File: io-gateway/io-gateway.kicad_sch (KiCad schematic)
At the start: 8 parts, among them J1 1752201, J2 1752201, J3 1752201, J4 Screw_Terminal_01x09, J5 Screw_Terminal_01x09, J6 Screw_Terminal_01x09

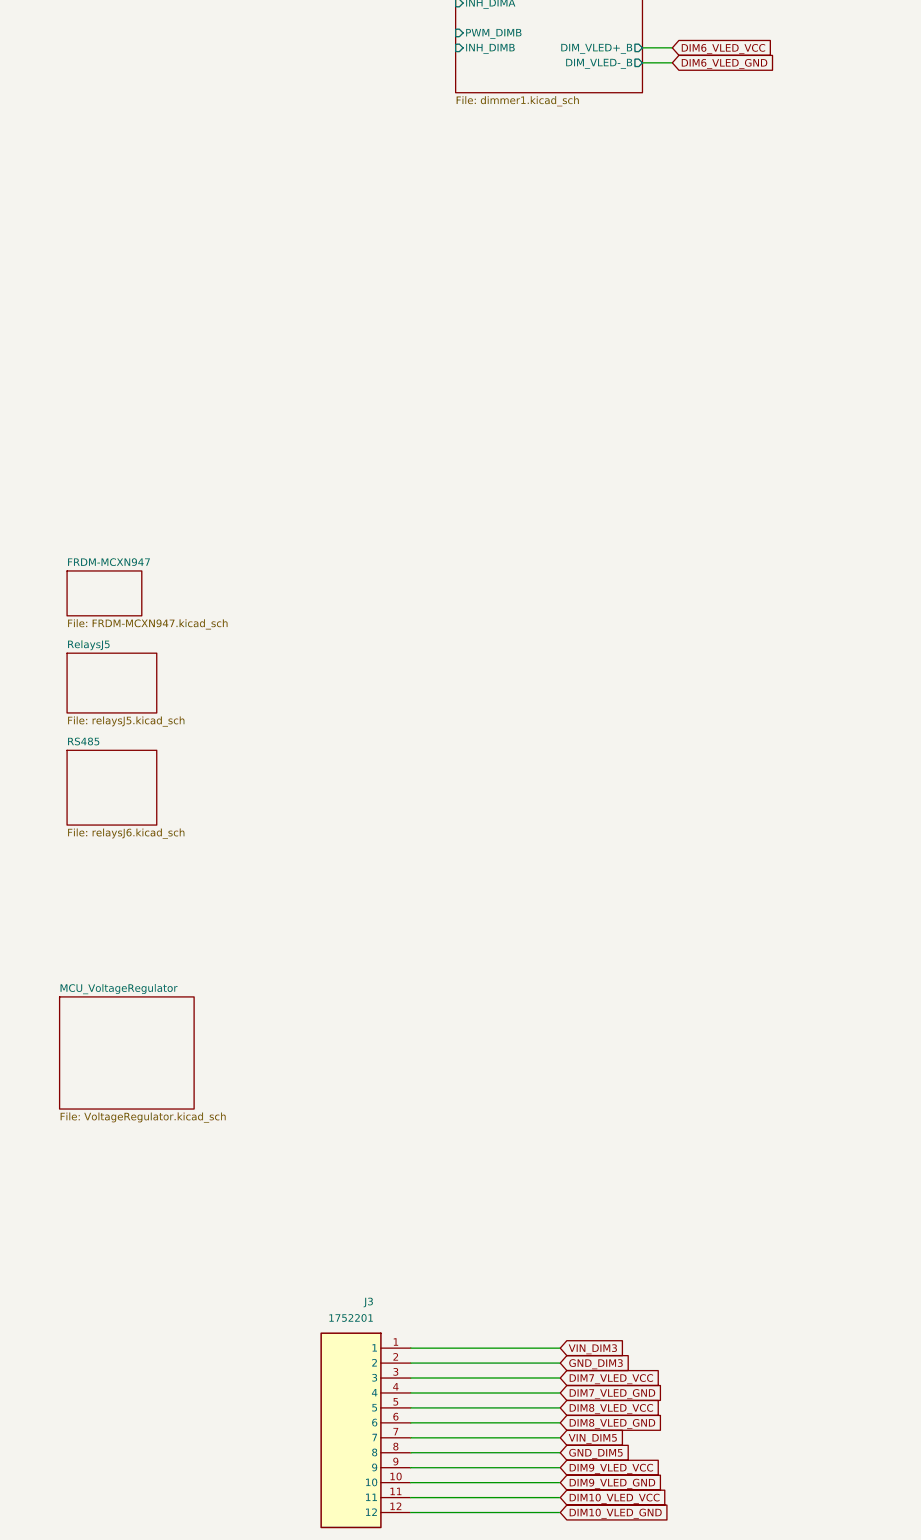
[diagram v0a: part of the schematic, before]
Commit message: upd
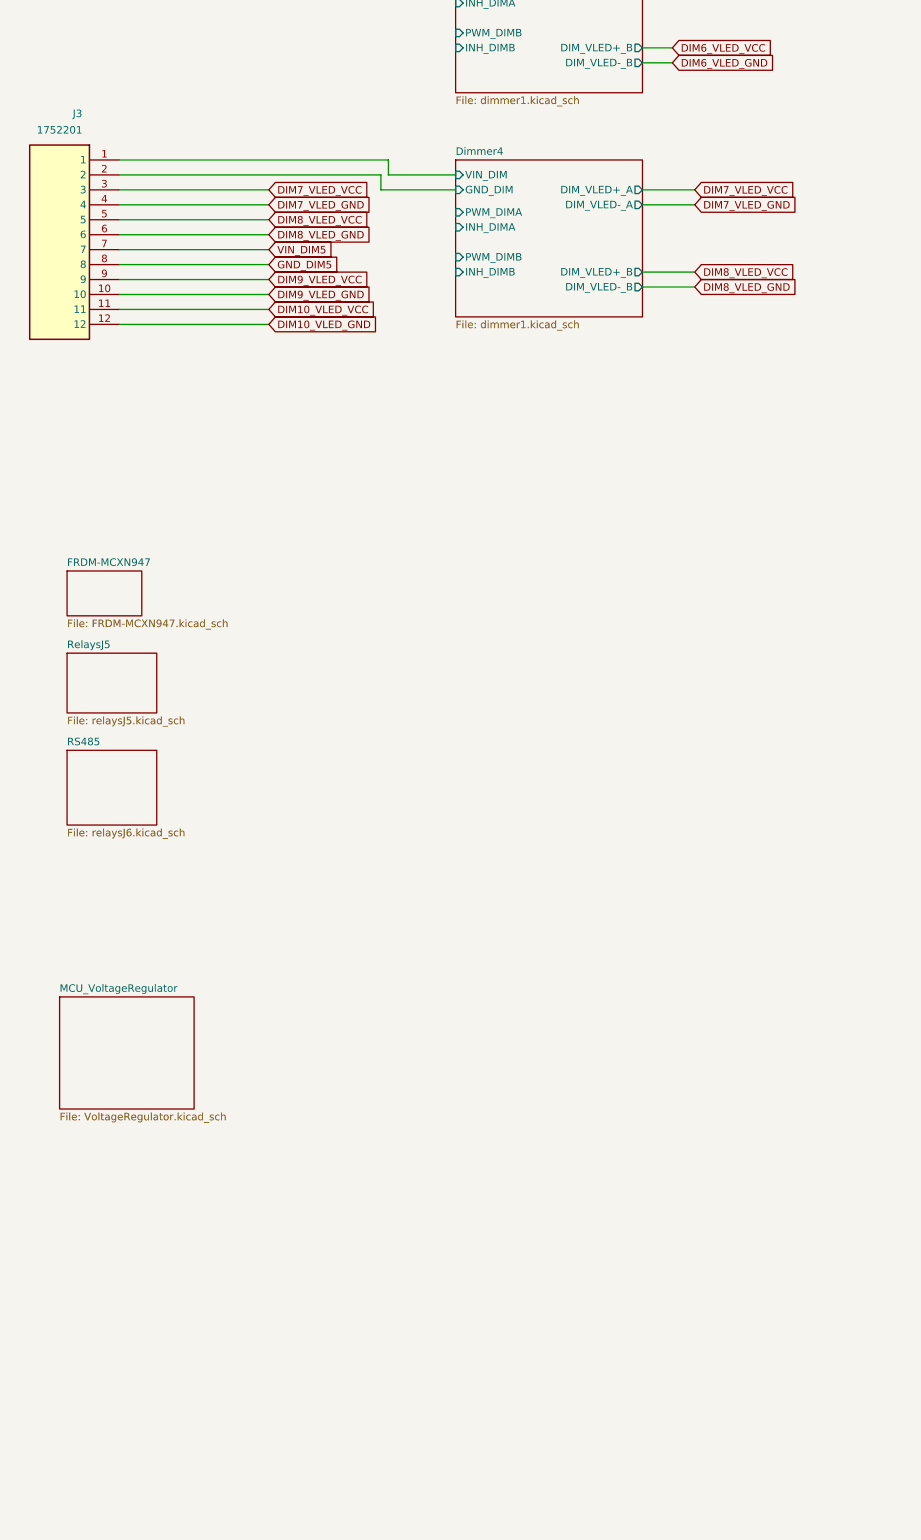
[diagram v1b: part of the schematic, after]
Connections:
- net GND_DIM3 renamed Dimmer4/GND_DIM
- net VIN_DIM3 renamed Dimmer4/VIN_DIM
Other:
- added sheet Dimmer4 (dimmer1.kicad_sch)
- moved on the sheet: J3
